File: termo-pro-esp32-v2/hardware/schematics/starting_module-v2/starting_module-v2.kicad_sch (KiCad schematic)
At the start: 17 parts, among them J1 Screw_Terminal_01x02, J2 Screw_Terminal_01x02, J3 Conn_01x08_Pin, K1 SANYOU_SRD_Form_C, Q1 PN2222A, SW2 SW_Push_LED, U2 ESP32-C3_SUPERMINI_TH

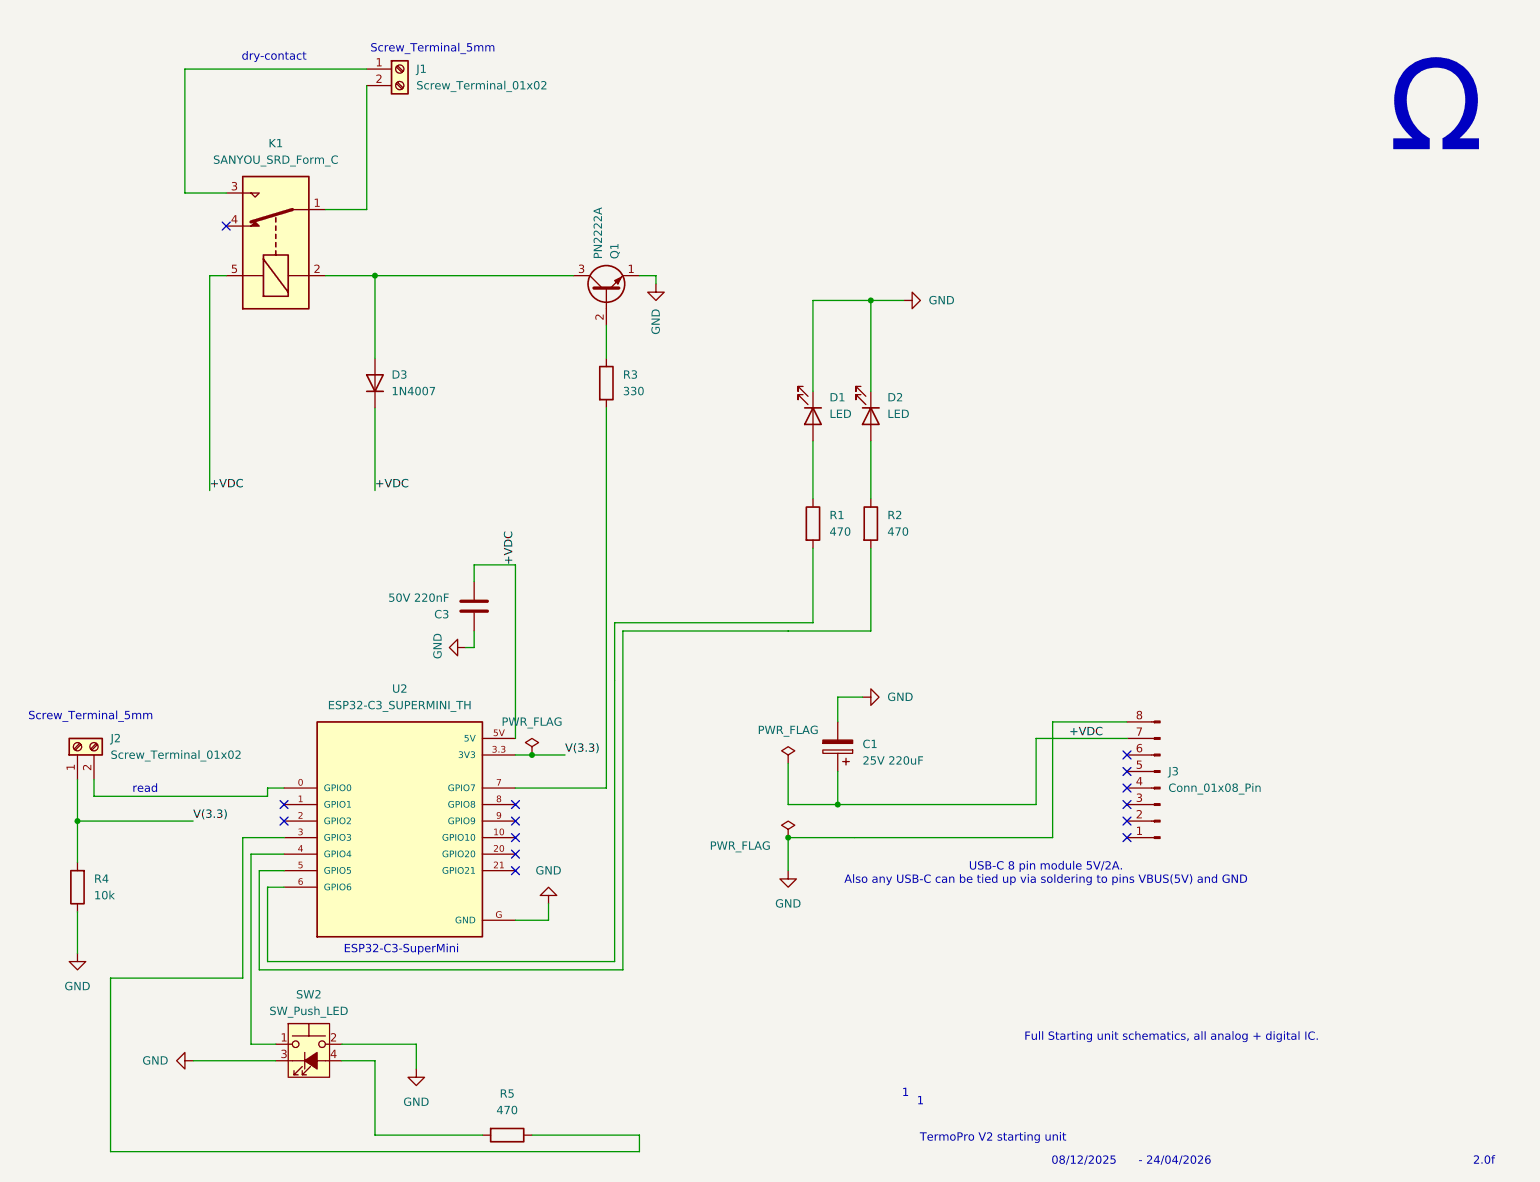
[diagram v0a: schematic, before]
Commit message: *
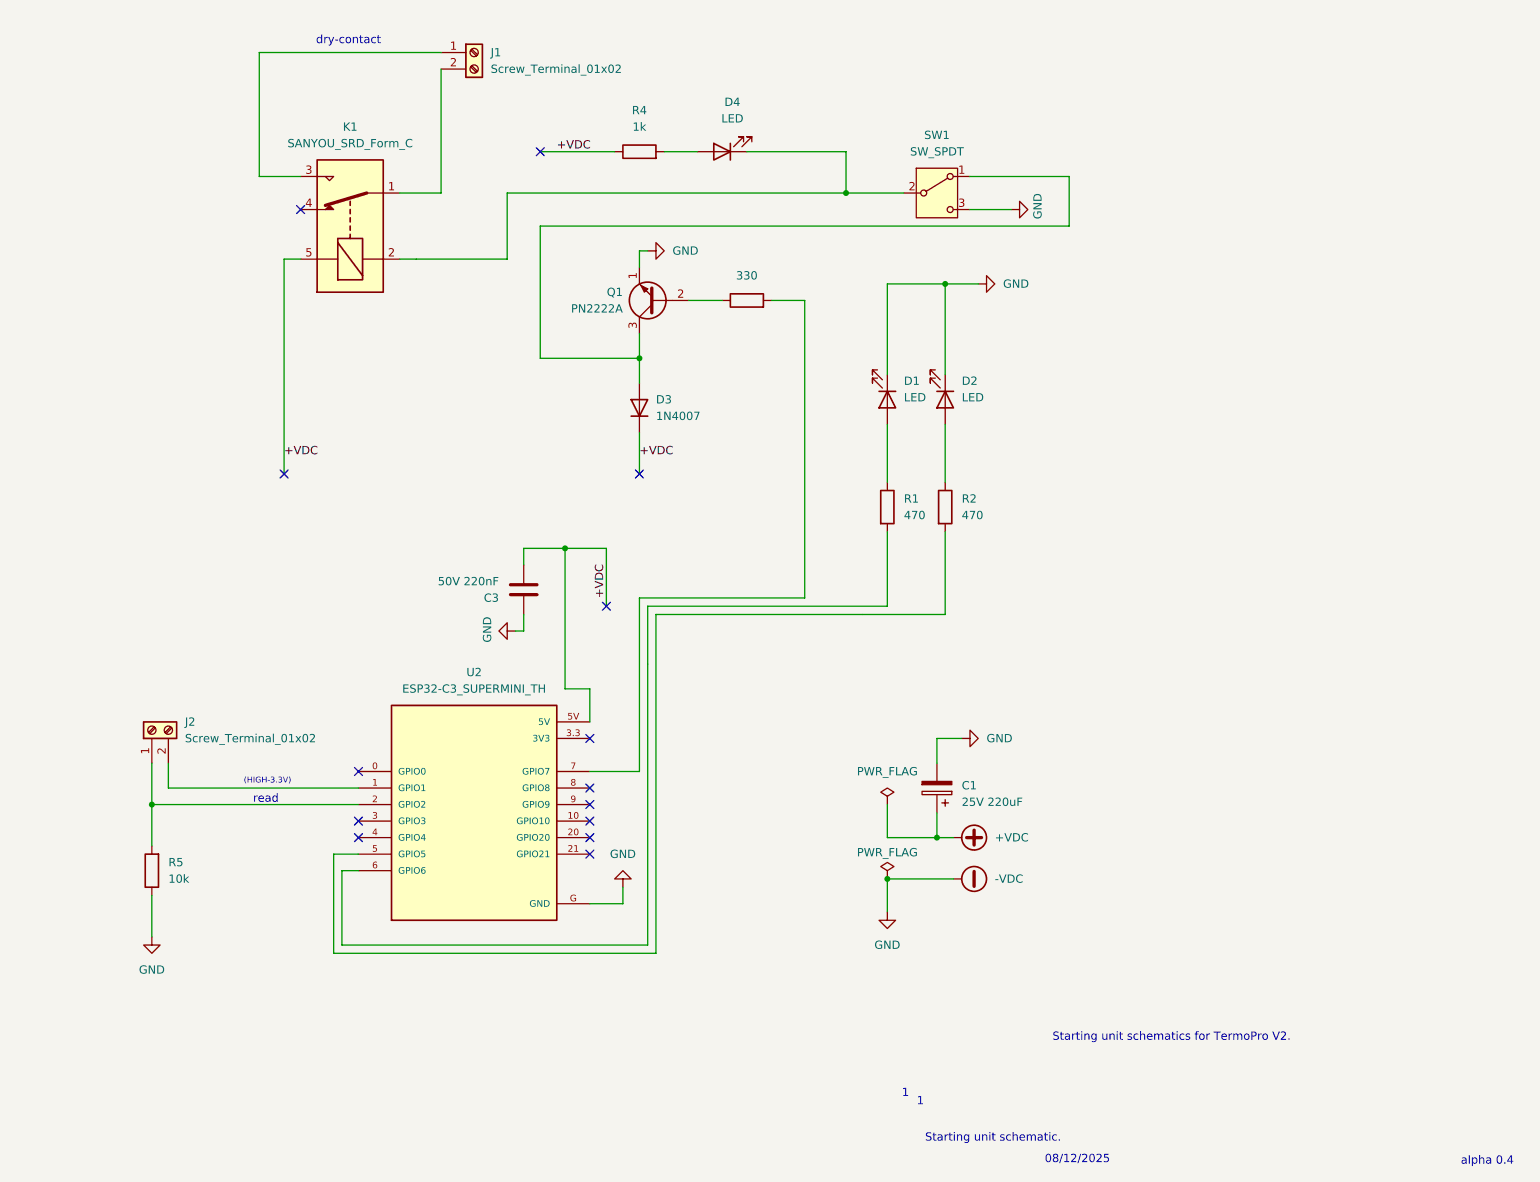
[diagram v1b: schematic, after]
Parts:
- removed J3: Conn_01x08_Pin, Connector_PinSocket_2.54mm:PinSocket_1x08_P2.54mm_Vertical, symbol Connector:Conn_01x08_Pin
- removed R5: 470, Resistor_THT:R_Axial_DIN0207_L6.3mm_D2.5mm_P10.16mm_Horizontal, symbol Device:R
- removed SW2: SW_Push_LED, SW_PUSH_THT_12mm:SW_PUSH-12mm, symbol Switch:SW_Push_LED
- added D4: LED, LED_THT:LED_D5.0mm_FlatTop, symbol Device:LED
- added R4: 1k, Resistor_THT:R_Axial_DIN0207_L6.3mm_D2.5mm_P7.62mm_Horizontal, symbol Device:R
- added SW1: SW_SPDT, Button_Switch_THT:SW_Slide_SPDT_Straight_CK_OS102011MS2Q, symbol Switch:SW_SPDT
- C3: footprint Capacitor_THT:C_Disc_D11.0mm_W5.0mm_P5.00mm -> Capacitor_THT:C_Radial_D10.0mm_H12.5mm_P5.00mm
- J1, J2: footprint TerminalBlock_RND:TerminalBlock_RND_205-00232_1x02_P5.08mm_Horizontal -> TerminalBlock_Phoenix:TerminalBlock_Phoenix_MKDS-1,5-2-5.08_1x02_P5.08mm_Horizontal
- R1, R2, R3: footprint Resistor_THT:R_Axial_DIN0207_L6.3mm_D2.5mm_P10.16mm_Horizontal -> Resistor_THT:R_Axial_DIN0207_L6.3mm_D2.5mm_P7.62mm_Horizontal
- R5: renamed from R4; footprint Resistor_THT:R_Axial_DIN0207_L6.3mm_D2.5mm_P10.16mm_Horizontal -> Resistor_THT:R_Axial_DIN0207_L6.3mm_D2.5mm_P7.62mm_Horizontal
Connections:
- net +VDC: now also R4.1
- net at D3.2 (A), Q1.3 (C): now also SW1.1 (A); no longer K1.2
- net at U2.0 (GPIO0): no longer J2.2 (Pin_2)
- net at U2.1 (GPIO1): now also J2.2 (Pin_2)
- net at U2.2 (GPIO2): now also J2.1 (Pin_1), R5.2
- net GND renamed -VDC
- net -VDC: now also SW1.3 (C)
- removed net V(3.3): J2.1 (Pin_1), R5.2, U2.3.3 (3V3)
- new net: D4.2 (A), R4.2
- new net: D4.1 (K), K1.2, SW1.2 (B)
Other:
- note added: "(HIGH-3.3V)"
- note added: "Starting unit schematic."
- note added: "Starting unit schematics for TermoPro V2."
- note added: "alpha 0.4"
- note removed: "- 24/04/2026"
- note removed: "2.0f"
- note removed: "ESP32-C3-SuperMini"
- note removed: "Full Starting unit schematics, all analog + digital IC."
- note removed: "Screw_Terminal_5mm"
- note removed: "TermoPro V2 starting unit"
- note removed: "USB-C 8 pin module 5V/2A. Also any USB-C can be tied up via soldering to pins VBUS(5V) and GND"
- note removed: "Ω"
- moved on the sheet: C1, C3, D1, D2, J1, J2, K1, Q1, R1, R2, R5, U2
